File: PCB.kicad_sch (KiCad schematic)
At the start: 14 parts

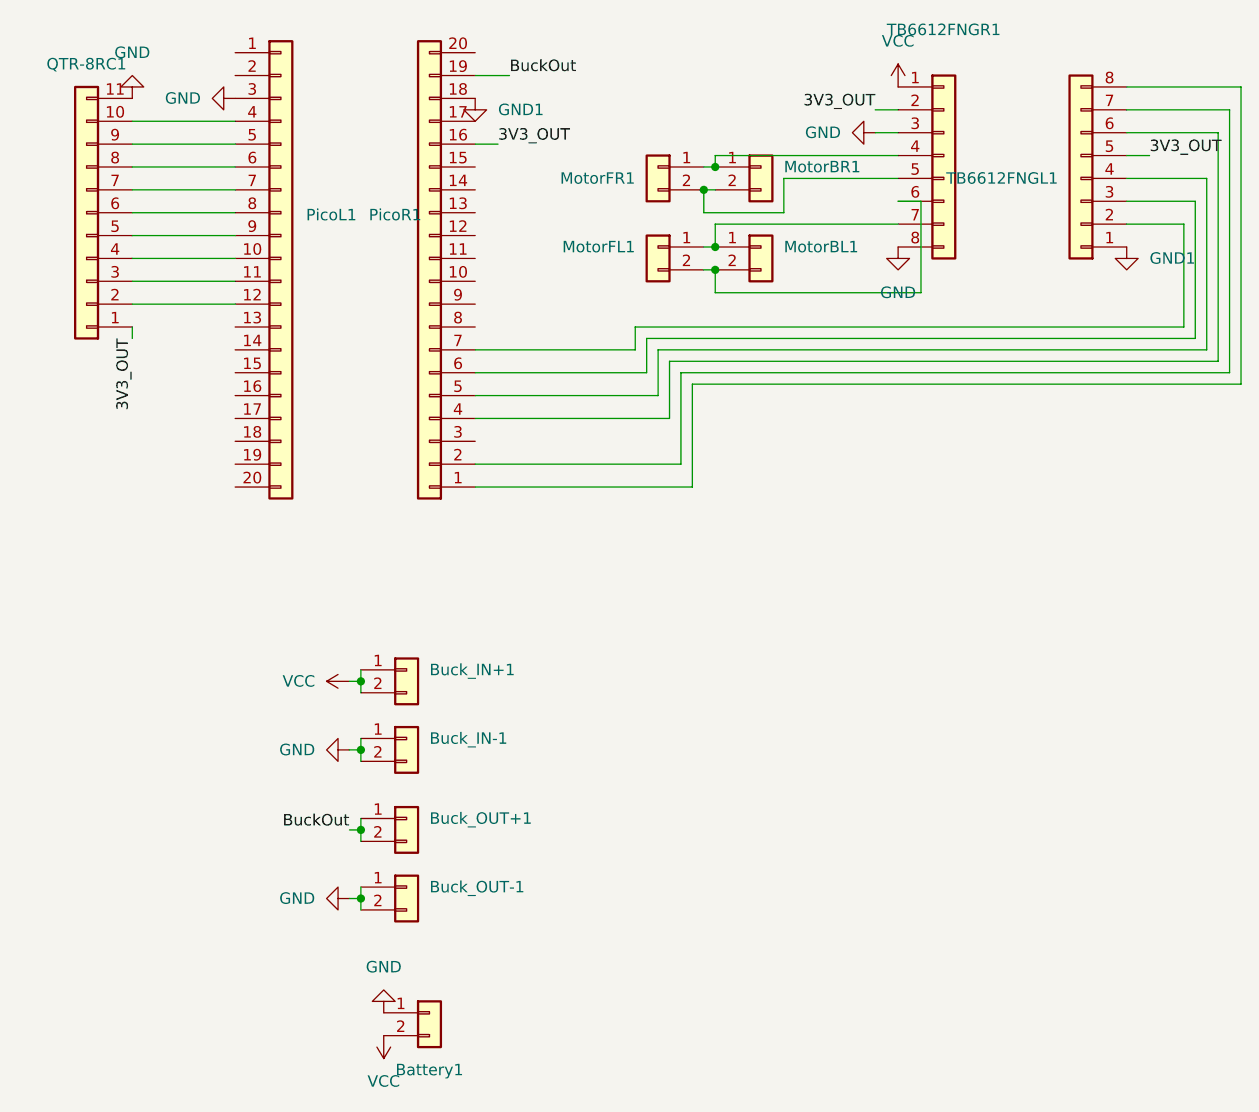
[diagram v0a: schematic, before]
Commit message: 3
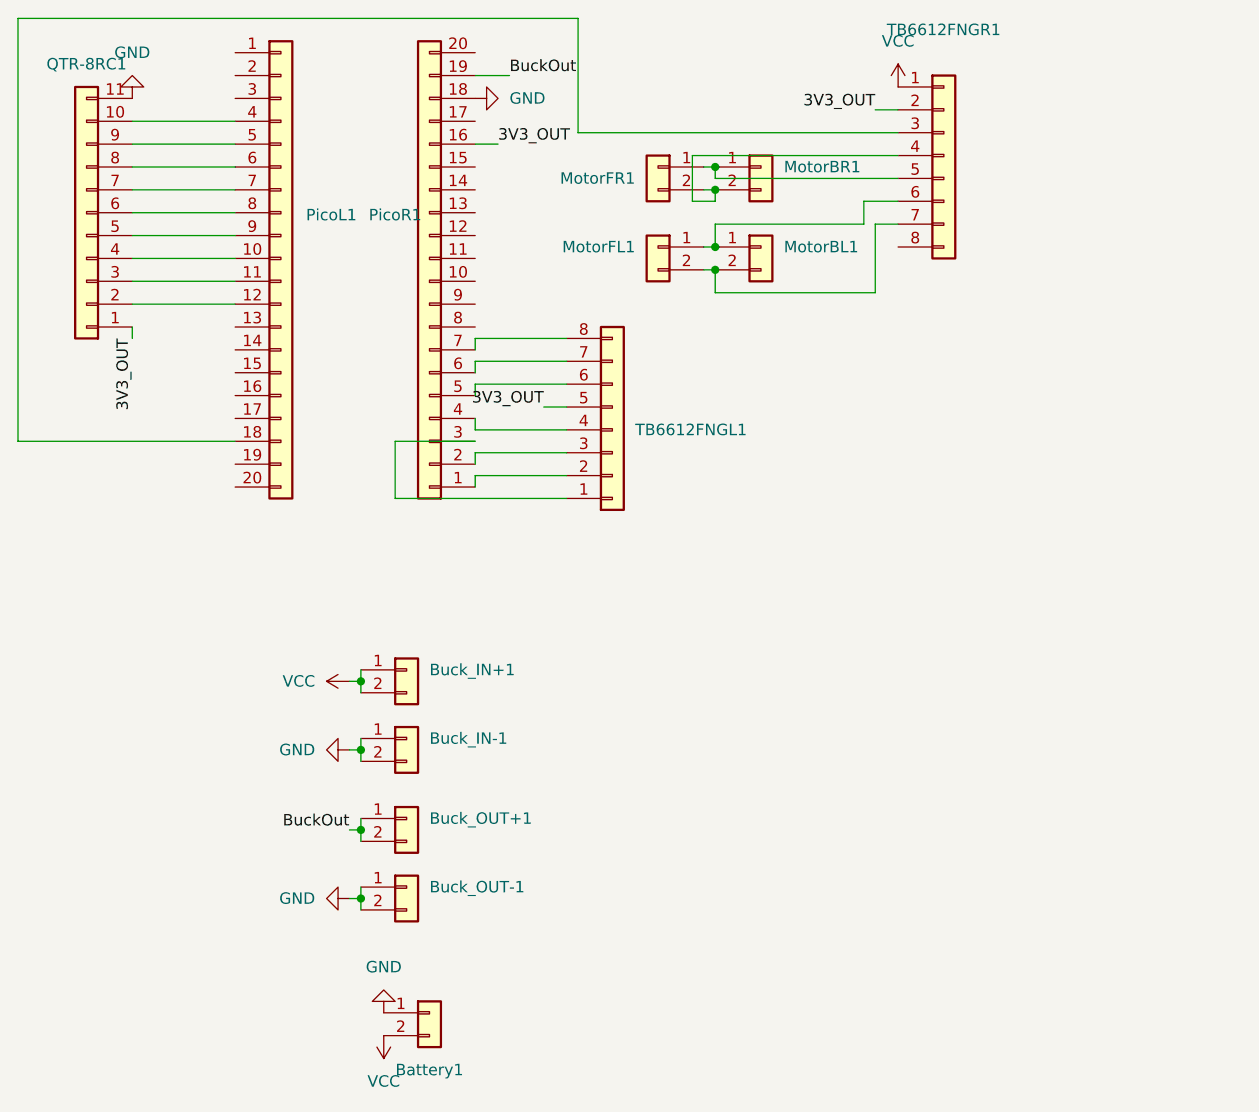
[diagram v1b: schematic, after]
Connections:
- net GND: now also PicoR1.18 (Pin_18); no longer PicoL1.3 (Pin_3), TB6612FNGR1.3 (Pin_3), TB6612FNGR1.8 (Pin_8)
- net at MotorBL1.1 (Pin_1), MotorFL1.1 (Pin_1): now also TB6612FNGR1.6 (Pin_6); no longer TB6612FNGR1.7 (Pin_7)
- net at MotorBL1.2 (Pin_2), MotorFL1.2 (Pin_2): now also TB6612FNGR1.7 (Pin_7); no longer TB6612FNGR1.6 (Pin_6)
- net at PicoR1.1 (Pin_1): now also TB6612FNGL1.2 (Pin_2); no longer TB6612FNGL1.8 (Pin_8)
- net at PicoR1.2 (Pin_2): now also TB6612FNGL1.3 (Pin_3); no longer TB6612FNGL1.7 (Pin_7)
- net at PicoR1.3 (Pin_3): now also TB6612FNGL1.1 (Pin_1)
- net at PicoR1.4 (Pin_4): now also TB6612FNGL1.4 (Pin_4); no longer TB6612FNGL1.6 (Pin_6)
- net at PicoR1.5 (Pin_5): now also TB6612FNGL1.6 (Pin_6); no longer TB6612FNGL1.4 (Pin_4)
- net at PicoR1.6 (Pin_6): now also TB6612FNGL1.7 (Pin_7); no longer TB6612FNGL1.3 (Pin_3)
- net at PicoR1.7 (Pin_7): now also TB6612FNGL1.8 (Pin_8); no longer TB6612FNGL1.2 (Pin_2)
- net at MotorBR1.1 (Pin_1), MotorFR1.1 (Pin_1): now also TB6612FNGR1.5 (Pin_5); no longer TB6612FNGR1.4 (Pin_4)
- net at MotorBR1.2 (Pin_2), MotorFR1.2 (Pin_2): now also TB6612FNGR1.4 (Pin_4); no longer TB6612FNGR1.5 (Pin_5)
- net at PicoL1.18 (Pin_18): now also TB6612FNGR1.3 (Pin_3)
- removed net GND1: PicoR1.18 (Pin_18), TB6612FNGL1.1 (Pin_1)
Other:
- moved on the sheet: TB6612FNGL1

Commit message: v1
1st completed version of PCB
Size is large than needed
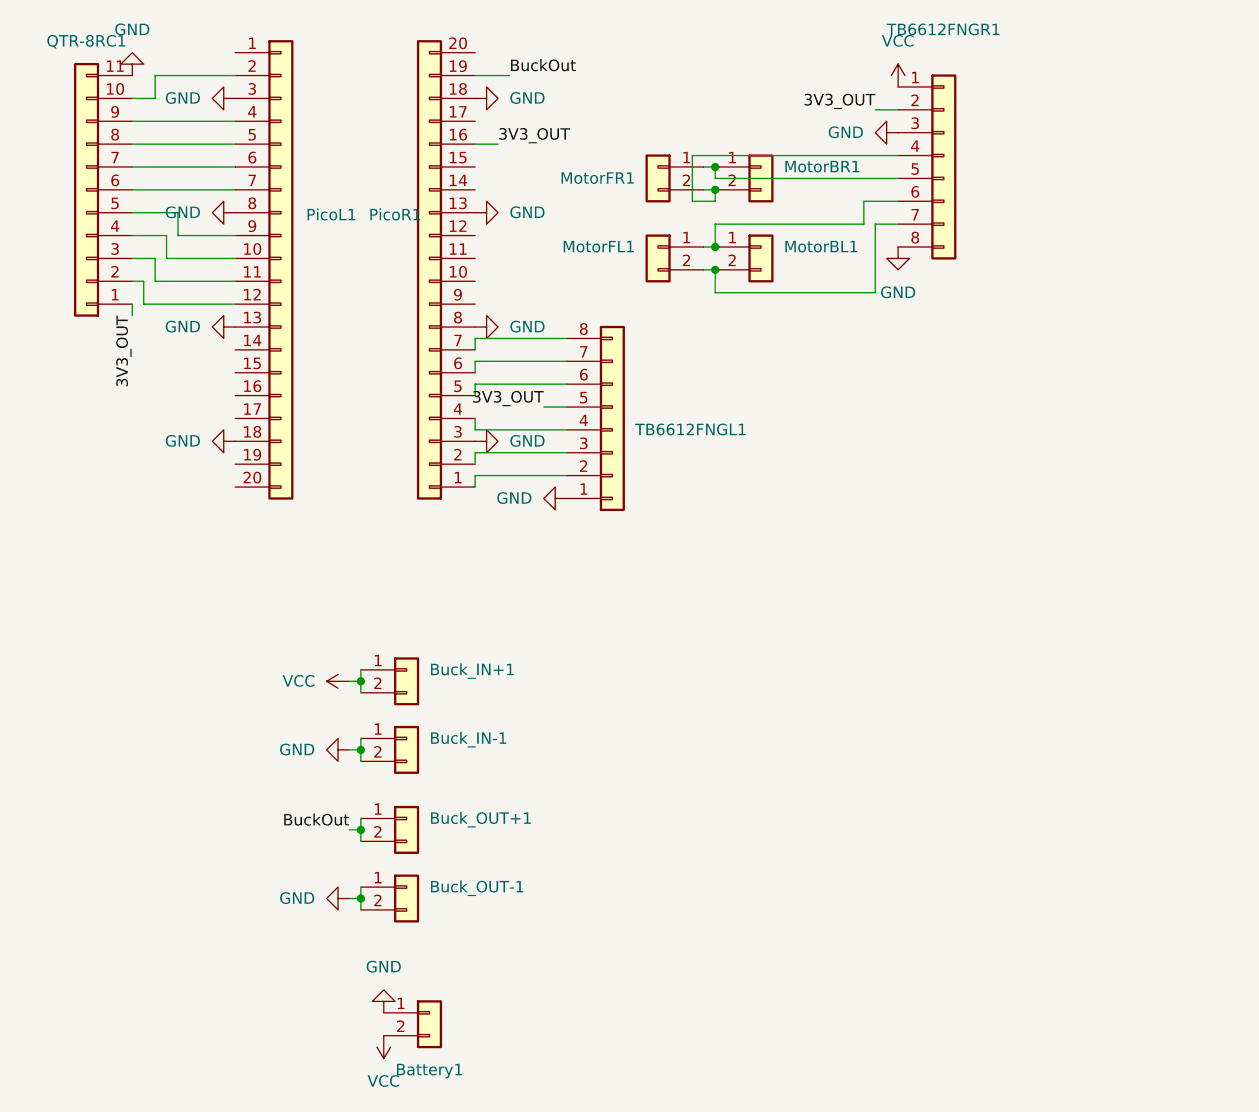
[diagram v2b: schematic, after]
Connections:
- net GND: now also PicoL1.13 (Pin_13), PicoL1.18 (Pin_18), PicoL1.3 (Pin_3), PicoL1.8 (Pin_8), PicoR1.13 (Pin_13), PicoR1.3 (Pin_3), PicoR1.8 (Pin_8), TB6612FNGL1.1 (Pin_1), TB6612FNGR1.3 (Pin_3), TB6612FNGR1.8 (Pin_8)
- net at QTR-8RC1.10 (Pin_10): now also PicoL1.2 (Pin_2); no longer PicoL1.4 (Pin_4)
- net at QTR-8RC1.6 (Pin_6): now also PicoL1.7 (Pin_7); no longer PicoL1.8 (Pin_8)
- net at QTR-8RC1.7 (Pin_7): now also PicoL1.6 (Pin_6); no longer PicoL1.7 (Pin_7)
- net at QTR-8RC1.8 (Pin_8): now also PicoL1.5 (Pin_5); no longer PicoL1.6 (Pin_6)
- net at QTR-8RC1.9 (Pin_9): now also PicoL1.4 (Pin_4); no longer PicoL1.5 (Pin_5)
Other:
- moved on the sheet: QTR-8RC1
